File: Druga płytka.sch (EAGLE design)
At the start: 6 parts, among them J1 826629-8, U1 MB85RS64V, U2 SCD40-D-R1

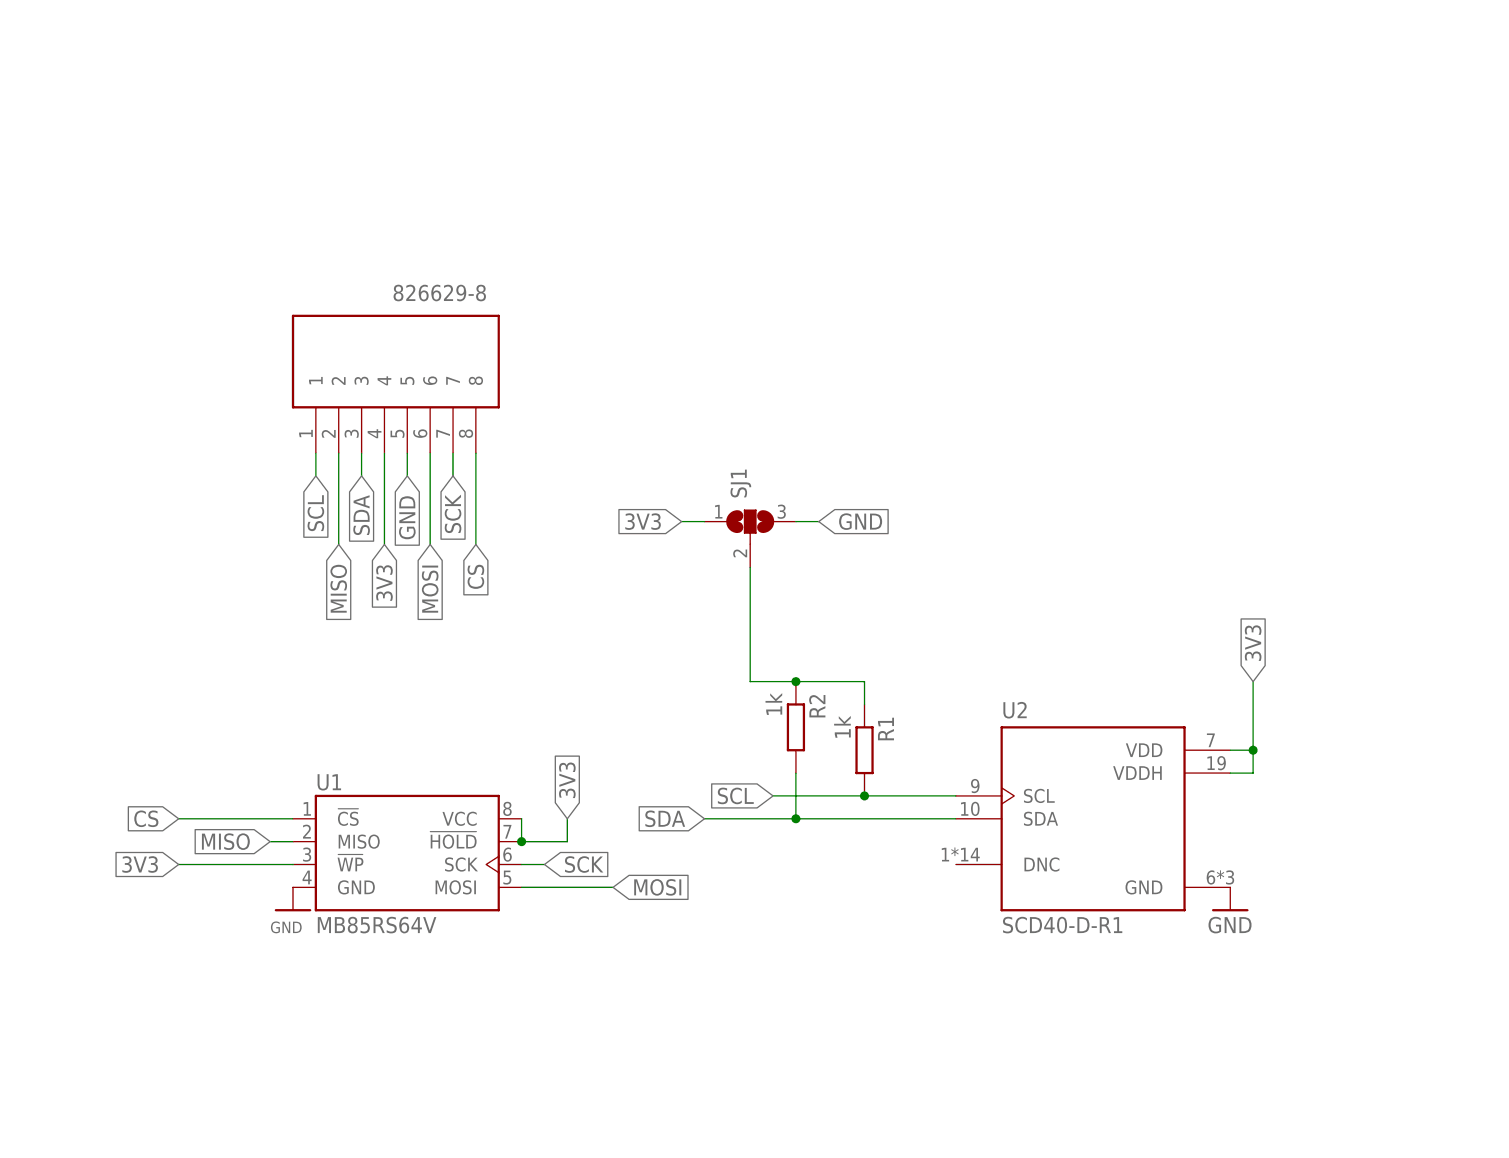
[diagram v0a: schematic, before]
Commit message: Add final project of PCB boards and cleaning repository up
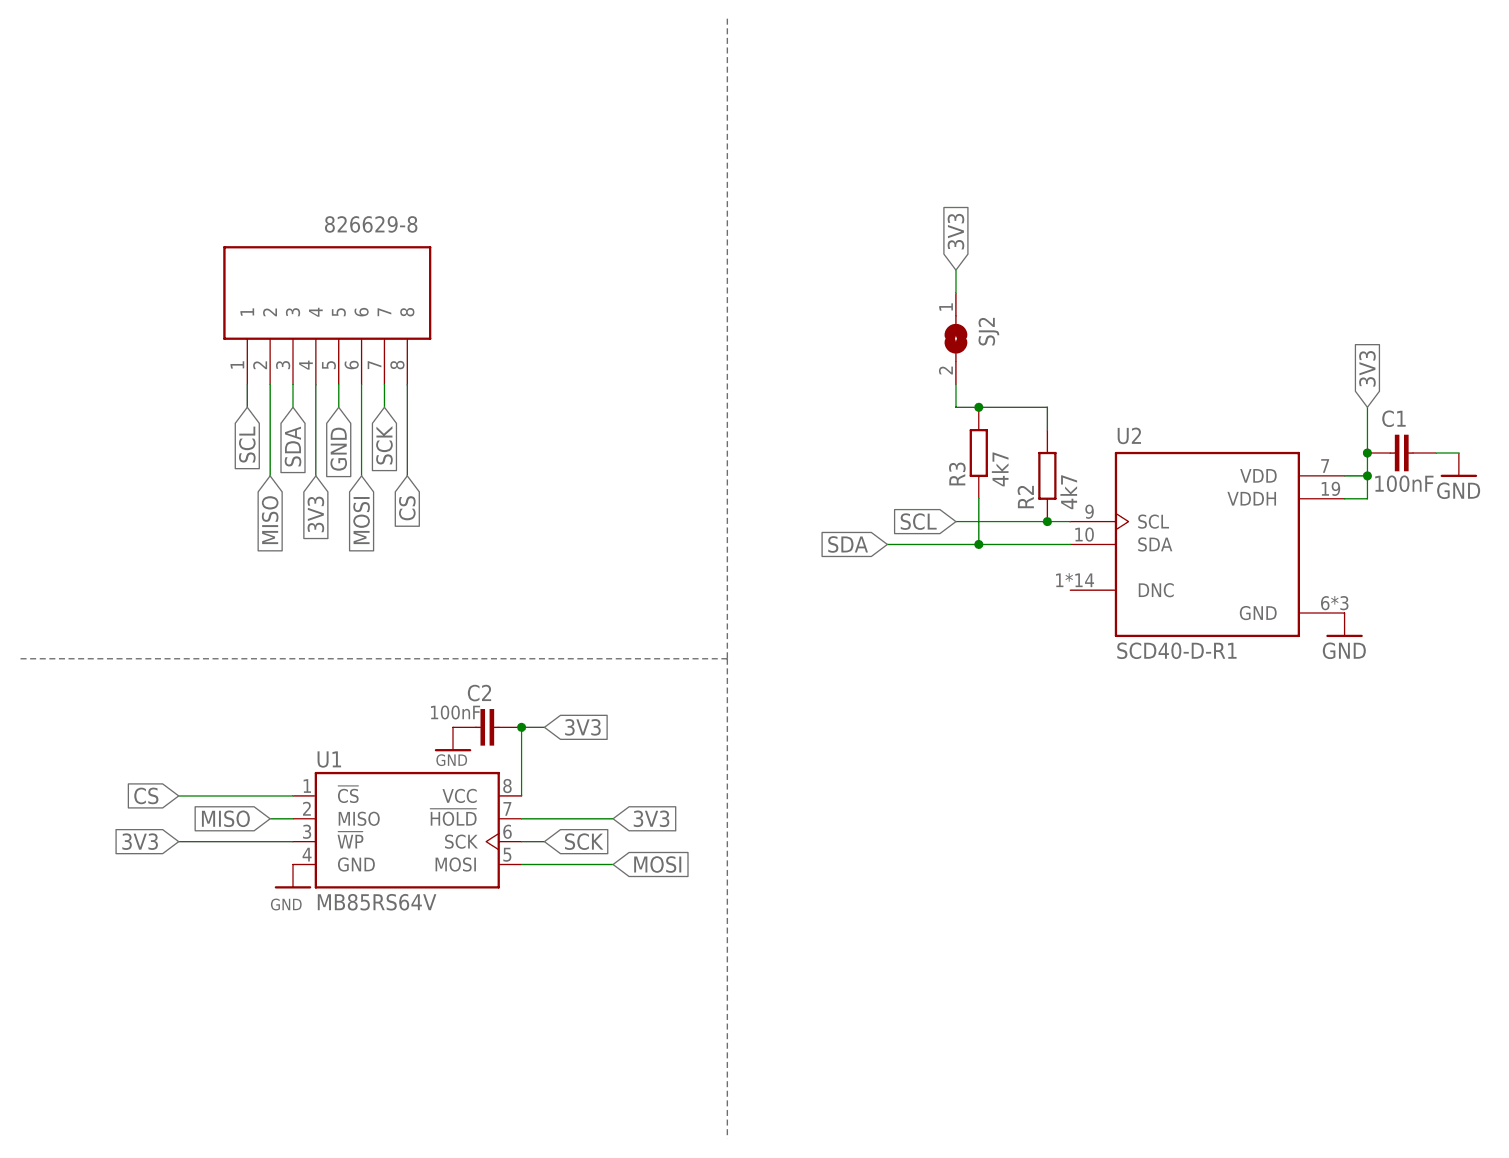
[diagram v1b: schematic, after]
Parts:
- removed R1: 1k, rcl:R-EU_0204/2V
- removed SJ1: (no value), jumper:SJ2W
- added C1, C2: 100nF, rcl:C-EUC0402
- added R3: 4k7, rcl:R-EU_R1206
- added SJ2: (no value), jumper:SJ
- R2: value 1k -> 4k7; device rcl:R-EU_0204/2V -> rcl:R-EU_R1206
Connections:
- net 3V3: now also C1.2, C2.1, SJ2.1; no longer SJ1.1
- net GND: now also C1.1, C2.2; no longer SJ1.3
- net JUMPER: now also R2.2, R3.2, SJ2.2; no longer R1.1, R2.1, SJ1.2
- net SCL: now also R2.1; no longer R1.2
- net SDA: now also R3.1; no longer R2.2
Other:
- moved on the sheet: R2, U1, U2
